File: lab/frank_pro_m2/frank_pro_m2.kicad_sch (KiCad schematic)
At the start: 18 parts, among them J1 UART, J2 DEBUG, J3 PWR

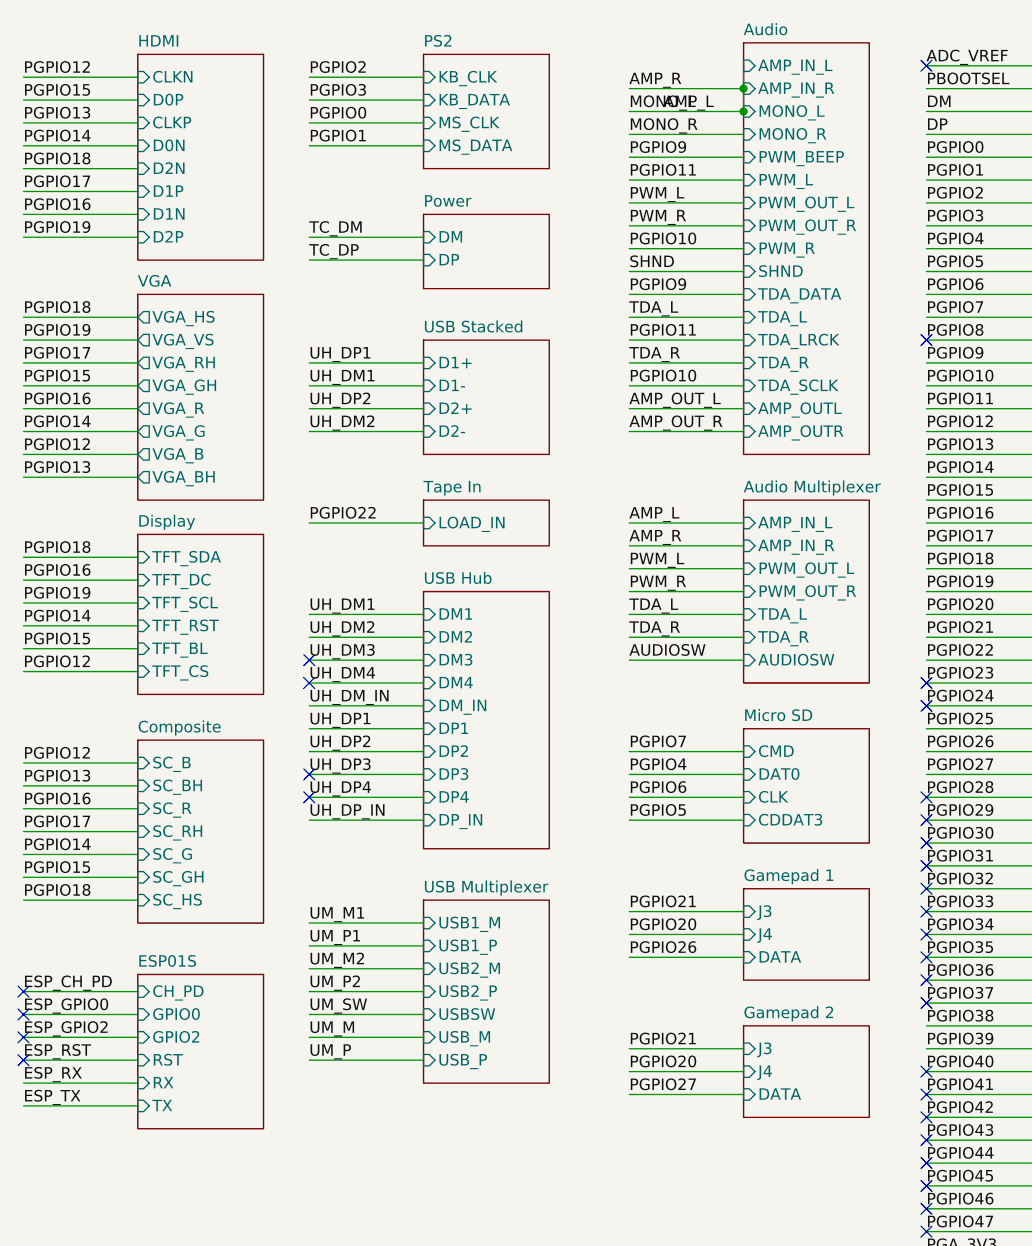
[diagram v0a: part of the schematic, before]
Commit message: Board updates
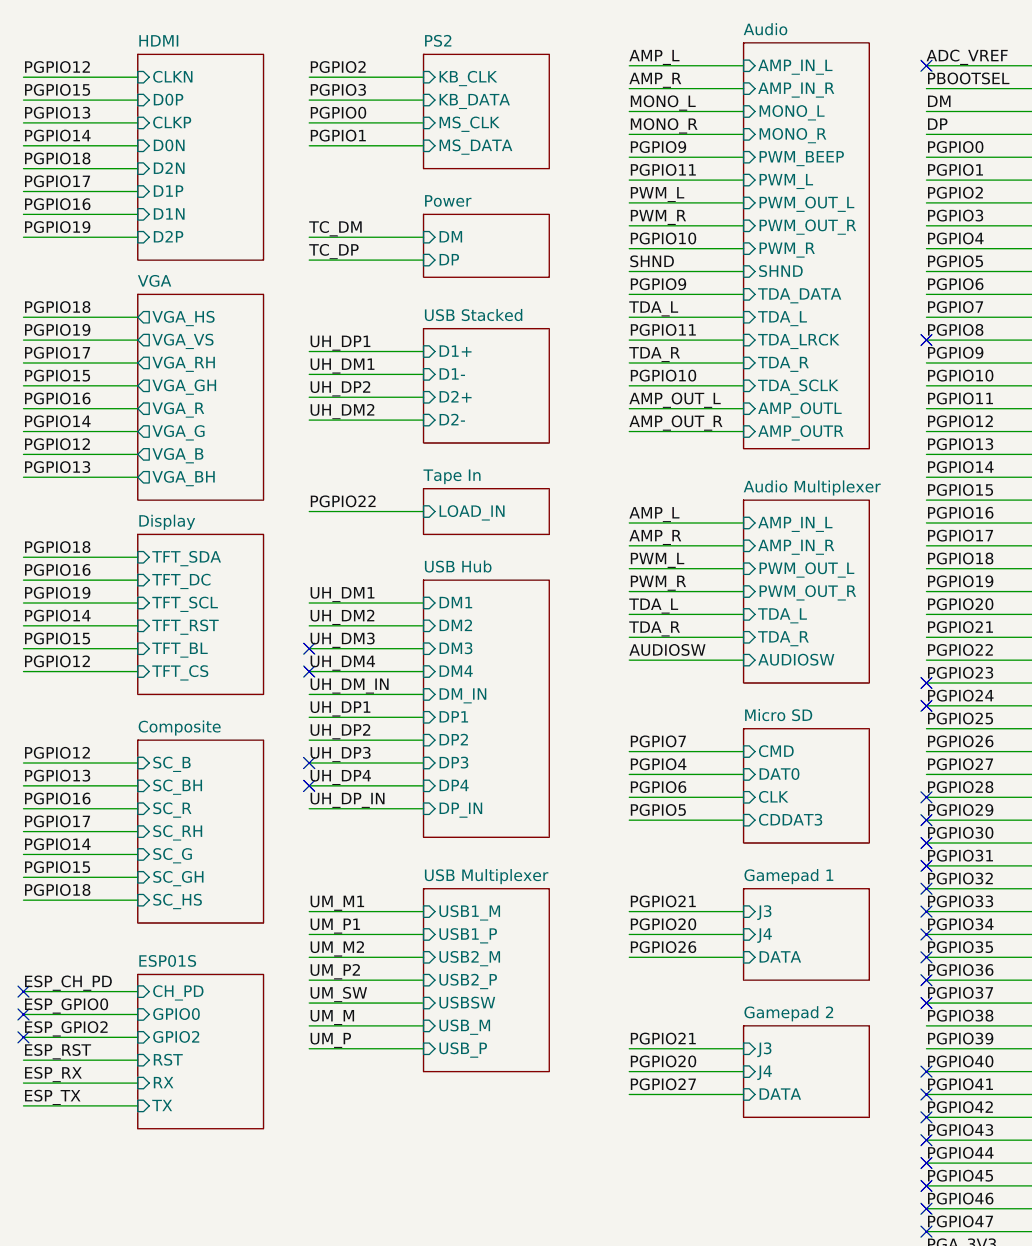
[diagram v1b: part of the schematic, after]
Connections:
- net AMP_L: no longer JP1.7 (COM_4)
- new net MONO_L: JP1.7 (COM_4)
- no-connect marks 33 -> 32
